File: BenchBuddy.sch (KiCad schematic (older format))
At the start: 0 parts

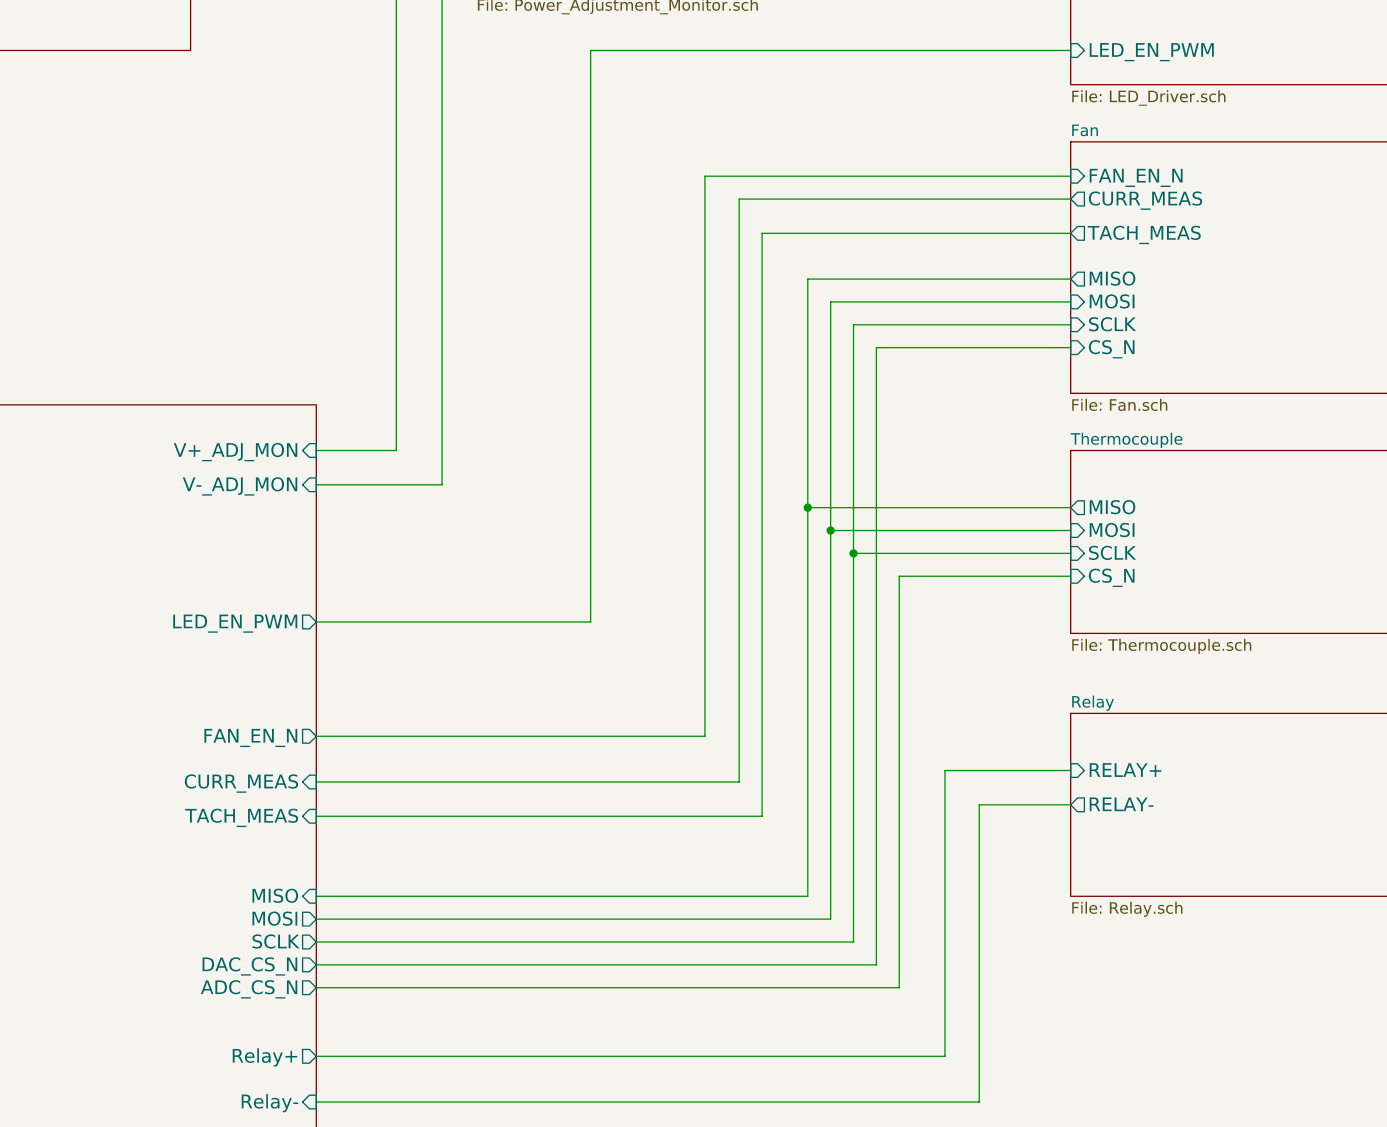
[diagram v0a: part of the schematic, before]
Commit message: Revisting the Current/Fan Module
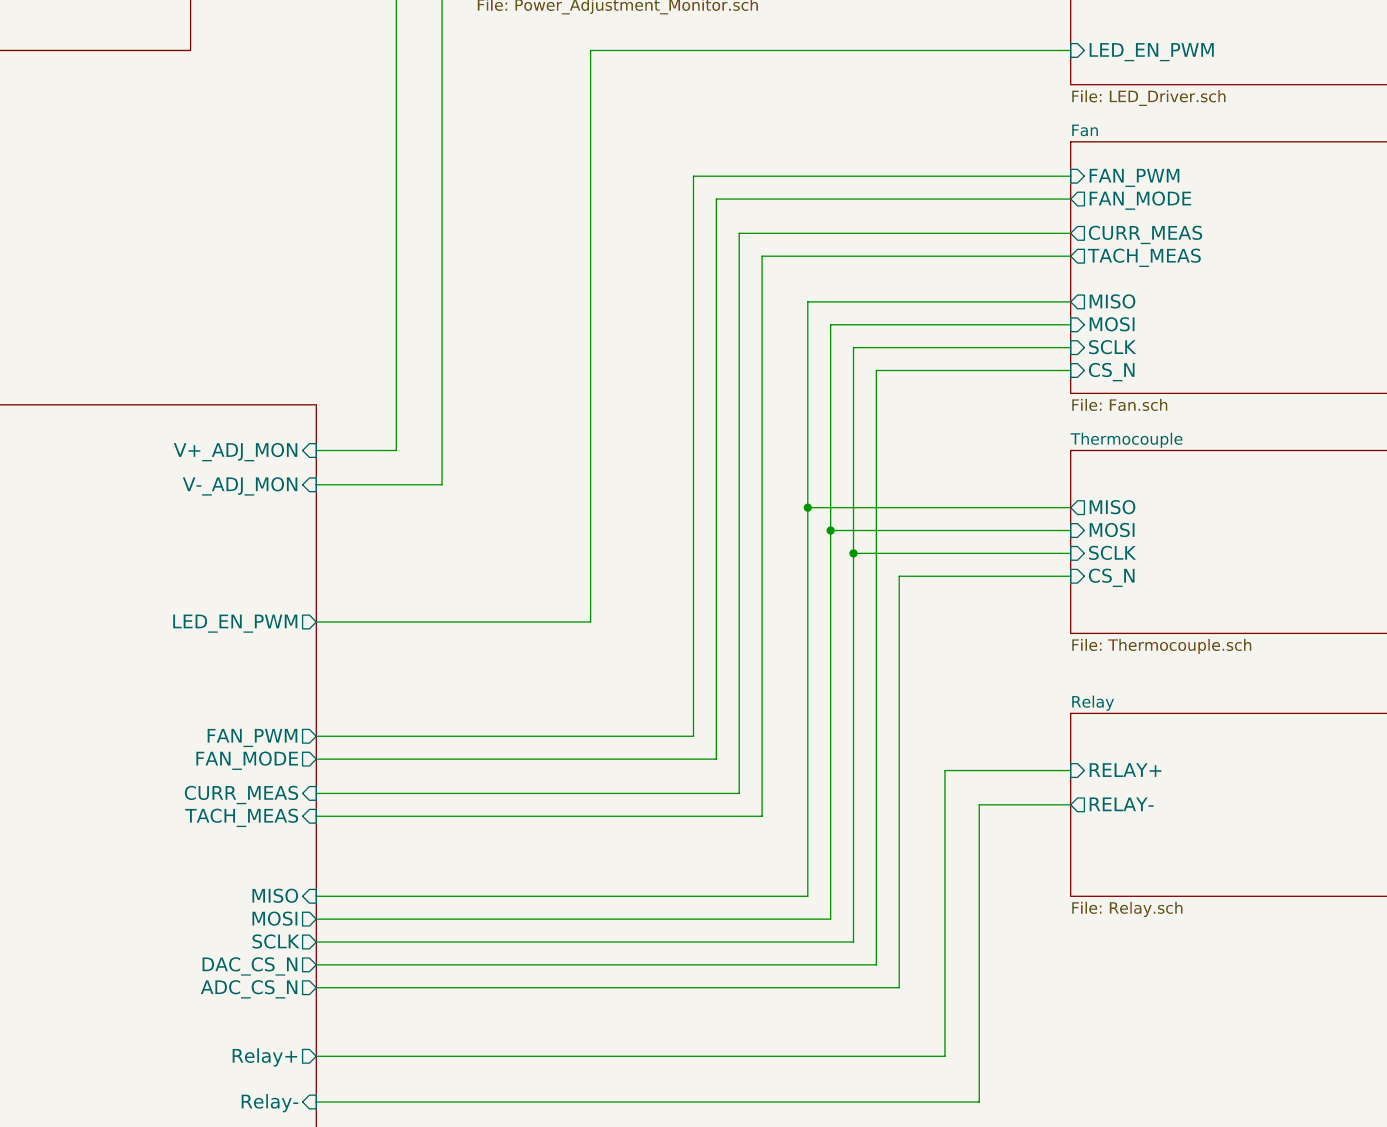
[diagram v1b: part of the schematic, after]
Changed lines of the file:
@@
 F5 "MISO" I R 3450 5950 60
 F6 "SCLK" O R 3450 6150 60
-F7 "FAN_EN_N" O R 3450 5250 60
-F8 "CURR_MEAS" I R 3450 5450 60
-F9 "LED_EN_PWM" O R 3450 4750 60
-F10 "TACH_MEAS" I R 3450 5600 60
-F11 "V+_ADJ_MON" I R 3450 4000 60
-F12 "V-_ADJ_MON" I R 3450 4150 60
-F13 "DAC_CS_N" O R 3450 6250 60
-F14 "ADC_CS_N" O R 3450 6350 60
+F7 "CURR_MEAS" I R 3450 5500 60
+F8 "LED_EN_PWM" O R 3450 4750 60
+F9 "TACH_MEAS" I R 3450 5600 60
+F10 "V+_ADJ_MON" I R 3450 4000 60
+F11 "V-_ADJ_MON" I R 3450 4150 60
+F12 "DAC_CS_N" O R 3450 6250 60
+F13 "ADC_CS_N" O R 3450 6350 60
+F14 "FAN_PWM" O R 3450 5250 60
+F15 "FAN_MODE" O R 3450 5350 60
 $EndSheet
 $Sheet
@@
 F0 "Fan" 50
 F1 "Fan.sch" 50
-F2 "MISO" O L 6750 3250 60
-F3 "MOSI" I L 6750 3350 60
-F4 "SCLK" I L 6750 3450 60
-F5 "CS_N" I L 6750 3550 60
+F2 "MISO" O L 6750 3350 60
+F3 "MOSI" I L 6750 3450 60
+F4 "SCLK" I L 6750 3550 60
+F5 "CS_N" I L 6750 3650 60
 F6 "FAN_OUT+" O R 8900 2850 60
 F7 "TACH_IN" I R 8900 3600 60
-F8 "TACH_MEAS" O L 6750 3050 60
-F9 "FAN_EN_N" I L 6750 2800 60
-F10 "CURR_MEAS" O L 6750 2900 60
-F11 "FAN_OUT-" O R 8900 3000 60
+F8 "TACH_MEAS" O L 6750 3150 60
+F9 "CURR_MEAS" O L 6750 3050 60
+F10 "FAN_OUT-" O R 8900 3000 60
+F11 "FAN_PWM" I L 6750 2800 60
+F12 "FAN_MODE" O L 6750 2900 60
 $EndSheet
 Wire Wire Line
@@
 	4650 4750 3450 4750
 Wire Wire Line
-	3450 5250 5150 5250
-Wire Wire Line
-	5150 5250 5150 2800
-Wire Wire Line
-	5150 2800 6750 2800
-Wire Wire Line
-	3450 5450 5300 5450
-Wire Wire Line
-	5300 5450 5300 2900
-Wire Wire Line
-	5300 2900 6750 2900
+	3450 5250 5100 5250
+Wire Wire Line
+	5100 5250 5100 2800
+Wire Wire Line
+	5100 2800 6750 2800
+Wire Wire Line
+	3450 5500 5300 5500
+Wire Wire Line
+	5300 5500 5300 3050
+Wire Wire Line
+	5300 3050 6750 3050
 Wire Wire Line
 	3450 5600 5400 5600
 Wire Wire Line
-	5400 5600 5400 3050
-Wire Wire Line
-	5400 3050 6750 3050
-Wire Wire Line
-	3450 5950 5600 5950
-Wire Wire Line
-	5600 5950 5600 4250
-Wire Wire Line
-	5600 4250 5600 3250
-Wire Wire Line
-	5600 3250 6750 3250
-Wire Wire Line
-	6750 3350 5700 3350
-Wire Wire Line
-	5700 3350 5700 4350
+	5400 5600 5400 3150
+Wire Wire Line
+	5400 3150 6750 3150
+Wire Wire Line
+	5600 5950 3450 5950
+Wire Wire Line
+	5600 3350 5600 4250
+Wire Wire Line
+	5600 4250 5600 5950
+Wire Wire Line
+	5600 3350 6750 3350
+Wire Wire Line
+	6750 3450 5700 3450
+Wire Wire Line
+	5700 3450 5700 4350
 Wire Wire Line
 	5700 4350 5700 6050
@@
 	5700 6050 3450 6050
 Wire Wire Line
-	3450 6150 5800 6150
-Wire Wire Line
-	5800 6150 5800 4450
-Wire Wire Line
-	5800 4450 5800 3450
-Wire Wire Line
-	5800 3450 6750 3450
+	5800 6150 3450 6150
+Wire Wire Line
+	5800 3550 5800 4450
+Wire Wire Line
+	5800 4450 5800 6150
+Wire Wire Line
+	5800 3550 6750 3550
 Wire Wire Line
 	6750 5400 6200 5400
@@
 	3450 6250 5900 6250
 Wire Wire Line
-	5900 6250 5900 3550
-Wire Wire Line
-	5900 3550 6750 3550
+	5900 6250 5900 3650
+Wire Wire Line
+	5900 3650 6750 3650
 Wire Wire Line
 	6750 4250 5600 4250
@@
 Wire Wire Line
 	6000 6350 3450 6350
+Wire Wire Line
+	6750 2900 5200 2900
+Wire Wire Line
+	5200 5350 5200 2900
+Wire Wire Line
+	3450 5350 5200 5350
 $EndSCHEMATC
